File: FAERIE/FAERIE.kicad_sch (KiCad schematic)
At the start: 35 parts, among them J1 UV Sensor, J10 12V IN, J11 Batt IN, J2 UV Bulb, J3 Sparkmax PWM, J4 Sparkmax, J5 Laser1, J7 CAN, J8 CAM1, J9 CAM2, Q1 SSM3K329R_LF, U1 D24V22Fx, U2 TJA1051T-3

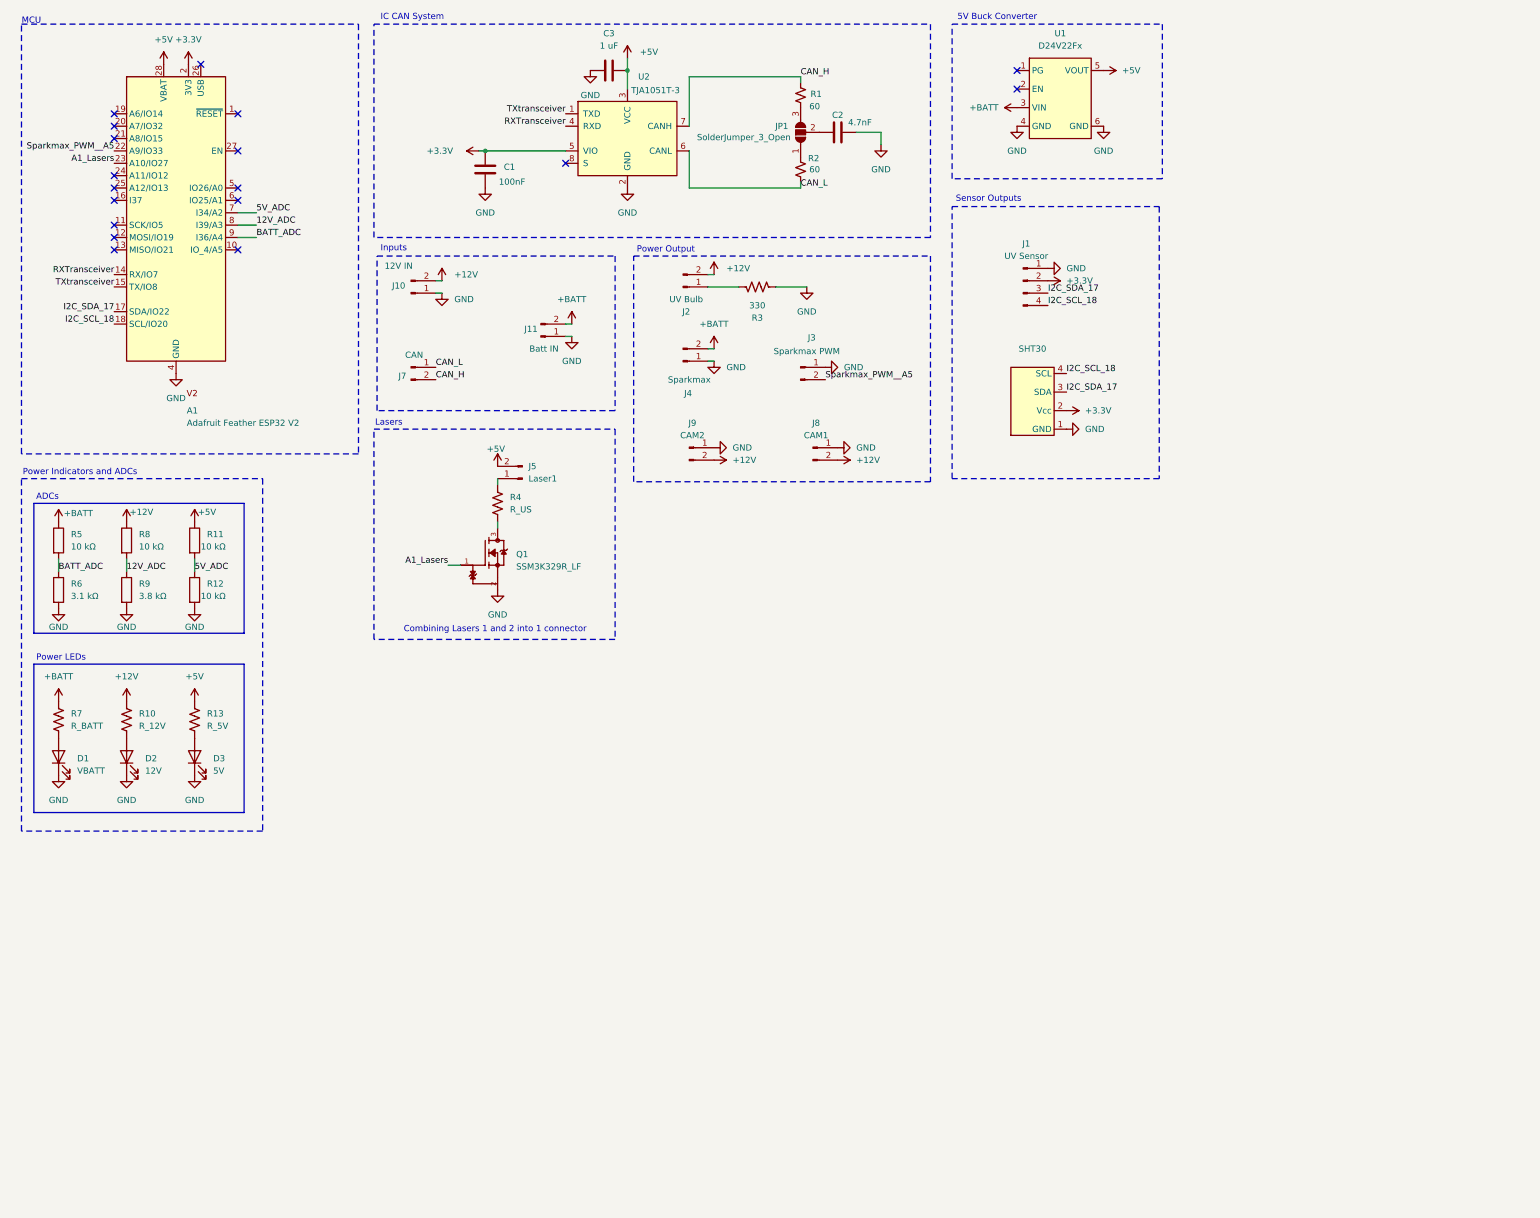
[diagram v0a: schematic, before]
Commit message: FAERIE 2026 V1
FAERIE April 15, 2026
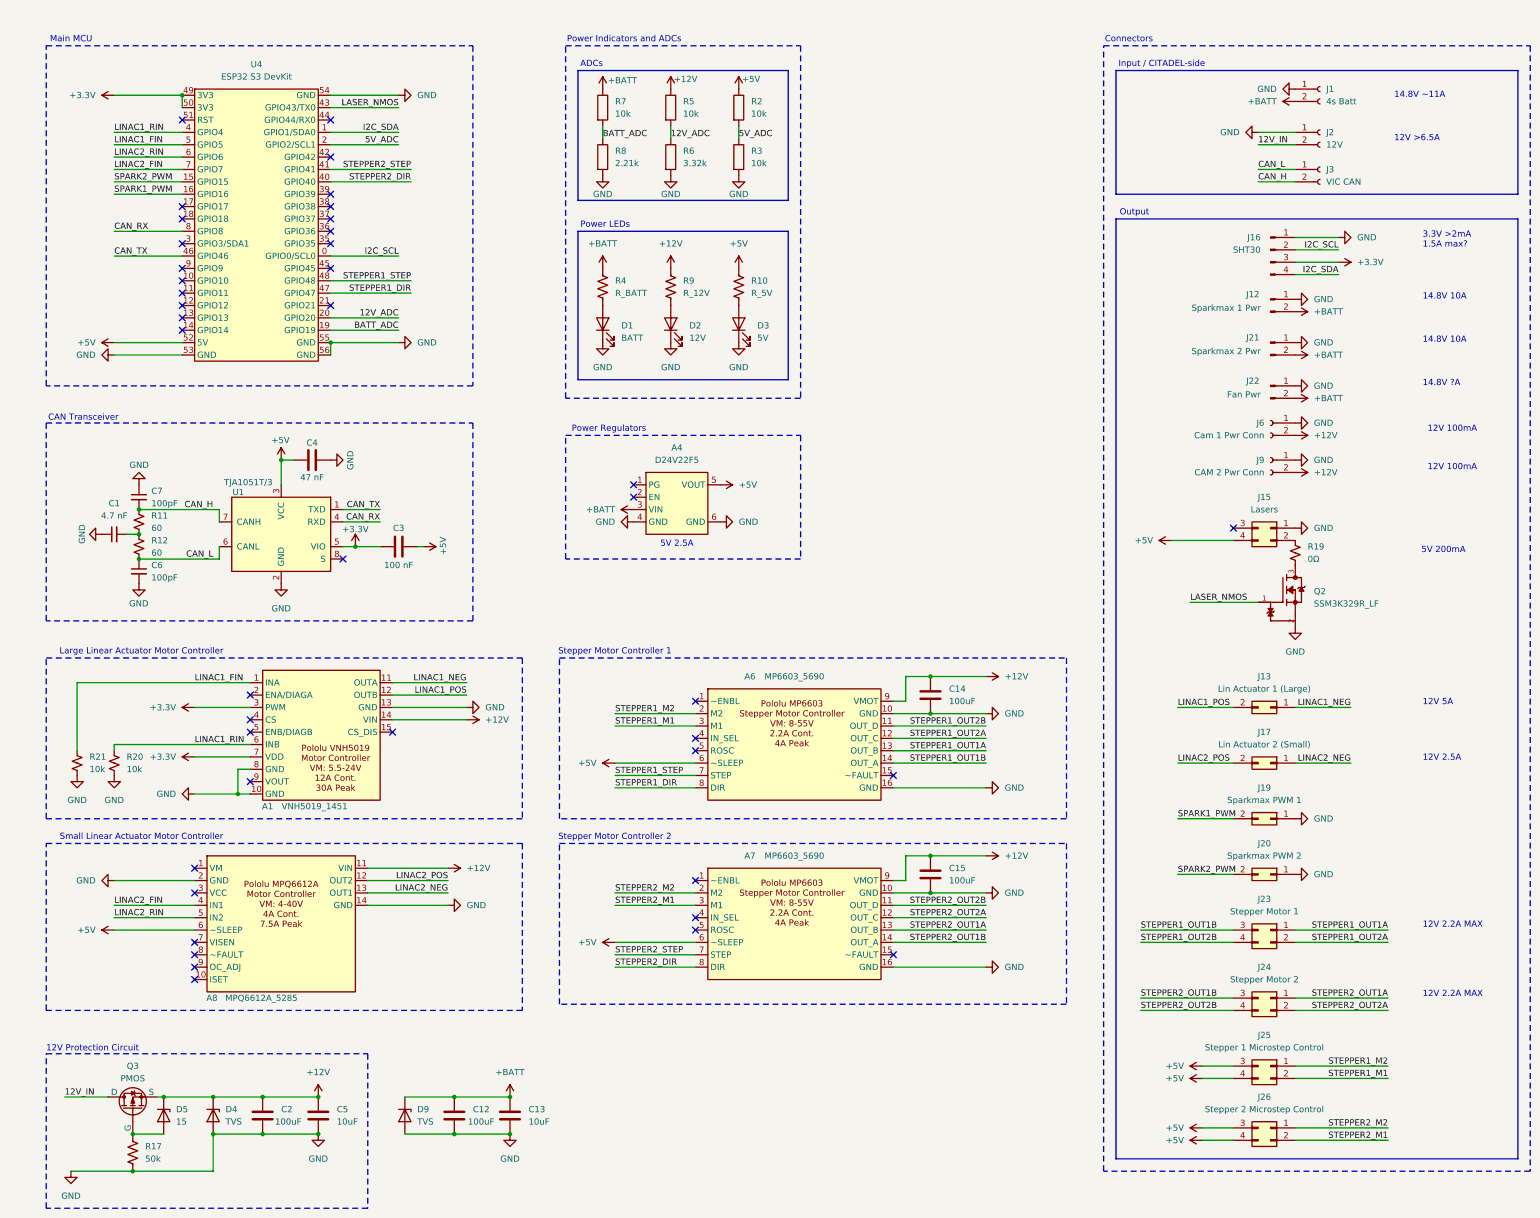
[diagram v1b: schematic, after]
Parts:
- removed A1: Adafruit Feather ESP32 V2, Module:Adafruit_Feather, symbol adafruit_feather_esp32_v2:Adafruit_Feather_ESP32_V2
- removed C1: 100nF, Capacitor_SMD:C_0603_1608Metric_Pad1.08x0.95mm_HandSolder, symbol Device:C
- removed J1: UV Sensor, Connector_Molex:Molex_Mini-Fit_Jr_5566-04A_2x02_P4.20mm_Vertical, symbol Connector:Conn_01x04_Pin
- removed J10: 12V IN, Connector_AMASS:AMASS_XT30PW-M_1x02_P2.50mm_Horizontal, symbol Connector:Conn_01x02_Pin
- removed J11: Batt IN, Connector_AMASS:AMASS_XT60PW-M_1x02_P7.20mm_Horizontal, symbol Connector:Conn_01x02_Pin
- removed J2: UV Bulb, Connector_Molex:Molex_Mini-Fit_Jr_5566-02A_2x01_P4.20mm_Vertical, symbol Connector:Conn_01x02_Pin
- removed J3: Sparkmax PWM, Connector_Molex:Molex_Mini-Fit_Jr_5566-02A_2x01_P4.20mm_Vertical, symbol Connector:Conn_01x02_Pin
- removed J4: Sparkmax, Connector_AMASS:AMASS_XT60PW-F_1x02_P7.20mm_Horizontal, symbol Connector:Conn_01x02_Pin
- removed J5: Laser1, Connector_Molex:Molex_Mini-Fit_Jr_5566-02A_2x01_P4.20mm_Vertical, symbol Connector:Conn_01x02_Pin
- removed J7: CAN, Connector_AMASS:AMASS_XT30PW-F_1x02_P2.50mm_Horizontal, symbol Connector:Conn_01x02_Pin
- removed J8: CAM1, Core_fp:XT30M_MODIFIED, symbol Connector:Conn_01x02_Pin
- removed J9: CAM2, Core_fp:XT30M_MODIFIED, symbol Connector:Conn_01x02_Pin
- removed JP1: SolderJumper_3_Open, Jumper:SolderJumper-3_P1.3mm_Open_Pad1.0x1.5mm_NumberLabels, symbol Jumper:SolderJumper_3_Open
- removed Q1: SSM3K329R_LF, Core_fp:SOTFL95P240X88-3N, symbol SSM3K329R_LF:SSM3K329R_LF
- removed R1, R2: 60, Resistor_SMD:R_0603_1608Metric_Pad0.98x0.95mm_HandSolder, symbol Device:R_Small_US
- removed R11, R12: 10 kΩ, Resistor_SMD:R_0603_1608Metric_Pad0.98x0.95mm_HandSolder, symbol Device:R
- removed R13: R_5V, Resistor_SMD:R_0603_1608Metric_Pad0.98x0.95mm_HandSolder, symbol Device:R_US
- removed R3: 330, Resistor_SMD:R_0603_1608Metric_Pad0.98x0.95mm_HandSolder, symbol Device:R_US
- removed R7: R_BATT, Resistor_SMD:R_0603_1608Metric_Pad0.98x0.95mm_HandSolder, symbol Device:R_US
- removed R9: 3.8 kΩ, Resistor_SMD:R_0603_1608Metric_Pad0.98x0.95mm_HandSolder, symbol Device:R
- removed SHT30: ~, Connector_Molex:Molex_Mini-Fit_Jr_5566-04A_2x02_P4.20mm_Vertical, symbol FAERIESYMBOLS:SHT30
- removed U1: D24V22Fx, Core_fp:D24V22Fx, symbol Core_sym:D24V22Fx
- removed U2: TJA1051T-3, Package_SO:SOIC-8_3.9x4.9mm_P1.27mm, symbol Interface_CAN_LIN:TJA1051T-3
- added A1: VNH5019_1451, FAERIE:VNH5019_1451, symbol Polulu:VNH5019_1451
- added A4: D24V22F5, FAERIE:D24V22Fx, symbol D24V22Fx:D24V22Fx
- added A6, A7: MP6603_5690, FAERIE:MP6603-5690, symbol Polulu:MP6603_5690
- added A8: MPQ6612A_5285, FAERIE:MPQ6612A_5285, symbol Polulu:MPQ6612A_5285
- added C1: 4.7 nF, Capacitor_SMD:C_0603_1608Metric_Pad1.08x0.95mm_HandSolder, symbol Device:C_Small
- added C12, C14, C15: 100uF, Capacitor_SMD:C_1210_3225Metric_Pad1.33x2.70mm_HandSolder, symbol Device:C
- added C13, C5: 10uF, Capacitor_SMD:C_0603_1608Metric_Pad1.08x0.95mm_HandSolder, symbol Device:C
- added C4: 47 nF, Capacitor_SMD:C_0603_1608Metric_Pad1.08x0.95mm_HandSolder, symbol Device:C
- added C6, C7: 100pF, Capacitor_SMD:C_0603_1608Metric_Pad1.08x0.95mm_HandSolder, symbol Device:C_Small
- added D4, D9: TVS, FAERIE:SOD-323HEUS2H_TOS, symbol Device:D_Zener
- added D5: 15, Diode_SMD:D_SOD-123, symbol Device:D_Zener
- added J1: 4s Batt, Connector_AMASS:AMASS_XT60PW-M_1x02_P7.20mm_Horizontal, symbol Connector:Conn_01x02_Socket
- added J12: Sparkmax 1 Pwr, Connector_AMASS:AMASS_XT60PW-F_1x02_P7.20mm_Horizontal, symbol Connector:Conn_01x02_Pin
- added J13: Lin Actuator 1 (Large), Connector_AMASS:AMASS_XT30U-F_1x02_P5.0mm_Vertical, symbol Connector_Generic:Conn_02x01
- added J15: Lasers, Connector_Molex:Molex_Mini-Fit_Jr_5566-04A_2x02_P4.20mm_Vertical, symbol Connector_Generic:Conn_02x02_Top_Bottom
- added J16: SHT30, Connector_Molex:Molex_Mini-Fit_Jr_5566-04A_2x02_P4.20mm_Vertical, symbol Connector:Conn_01x04_Pin
- added J17: Lin Actuator 2 (Small), Connector_AMASS:AMASS_XT30U-F_1x02_P5.0mm_Vertical, symbol Connector_Generic:Conn_02x01
- added J19: Sparkmax PWM 1, Connector_AMASS:AMASS_XT30U-F_1x02_P5.0mm_Vertical, symbol Connector_Generic:Conn_02x01
- added J2: 12V, Connector_AMASS:AMASS_XT30PW-M_1x02_P2.50mm_Horizontal, symbol Connector:Conn_01x02_Socket
- added J20: Sparkmax PWM 2, Connector_AMASS:AMASS_XT30U-F_1x02_P5.0mm_Vertical, symbol Connector_Generic:Conn_02x01
- added J21: Sparkmax 2 Pwr, Connector_AMASS:AMASS_XT60PW-F_1x02_P7.20mm_Horizontal, symbol Connector:Conn_01x02_Pin
- added J22: Fan Pwr, Connector_AMASS:AMASS_XT60PW-F_1x02_P7.20mm_Horizontal, symbol Connector:Conn_01x02_Pin
- added J23: Stepper Motor 1, Connector_Molex:Molex_Mini-Fit_Jr_5566-04A_2x02_P4.20mm_Vertical, symbol Connector_Generic:Conn_02x02_Top_Bottom
- added J24: Stepper Motor 2, Connector_Molex:Molex_Mini-Fit_Jr_5566-04A_2x02_P4.20mm_Vertical, symbol Connector_Generic:Conn_02x02_Top_Bottom
- added J25: Stepper 1 Microstep Control, Connector_PinHeader_2.54mm:PinHeader_2x02_P2.54mm_Vertical, symbol Connector_Generic:Conn_02x02_Top_Bottom
- added J26: Stepper 2 Microstep Control, Connector_PinHeader_2.54mm:PinHeader_2x02_P2.54mm_Vertical, symbol Connector_Generic:Conn_02x02_Top_Bottom
- added J3: VIC CAN, Connector_AMASS:AMASS_XT30PW-F_1x02_P2.50mm_Horizontal, symbol Connector:Conn_01x02_Socket
- added J6: Cam 1 Pwr Conn, Connector_AMASS:AMASS_XT30U-F_1x02_P5.0mm_Vertical, symbol Connector:Conn_01x02_Socket
- added J9: CAM 2 Pwr Conn, Connector_AMASS:AMASS_XT30U-F_1x02_P5.0mm_Vertical, symbol Connector:Conn_01x02_Socket
- added Q2: SSM3K329R_LF, FAERIE:SOT-23F_TOS, symbol SSM3K329R_LF:SSM3K329R_LF
- added Q3: PMOS, Package_TO_SOT_SMD:TO-252-2, symbol Simulation_SPICE:PMOS
- added R11, R12: 60, Resistor_SMD:R_0603_1608Metric_Pad0.98x0.95mm_HandSolder, symbol Device:R_Small_US
- added R17: 50k, Resistor_SMD:R_0603_1608Metric_Pad0.98x0.95mm_HandSolder, symbol Device:R_US
- added R19: 0Ω, Resistor_SMD:R_0603_1608Metric_Pad0.98x0.95mm_HandSolder, symbol Device:R_Small_US
- added R2, R3, R7: 10k, Resistor_SMD:R_0603_1608Metric_Pad0.98x0.95mm_HandSolder, symbol Device:R
- added R20, R21: 10k, Resistor_SMD:R_0603_1608Metric_Pad0.98x0.95mm_HandSolder, symbol Device:R_Small_US
- added R9: R_12V, Resistor_SMD:R_0603_1608Metric_Pad0.98x0.95mm_HandSolder, symbol Device:R_US
- added U1: TJA1051T/3, Package_SO:SOIC-8_3.9x4.9mm_P1.27mm, symbol Interface_CAN_LIN:TJA1051T-3
- added U4: ESP32 S3 DevKit, FAERIE:ESP32-S3-DevKit_No_Keep-Out_Zone, symbol SANXIXING:ESP32_S3_Dev_Board
- C2: value 4.7nF -> 100uF; footprint Capacitor_SMD:C_0603_1608Metric_Pad1.08x0.95mm_HandSolder -> Capacitor_SMD:C_1210_3225Metric_Pad1.33x2.70mm_HandSolder
- C3: value 1 uF -> 100 nF
- D1: value VBATT -> BATT
- R10: value R_12V -> R_5V
- R4: value R_US -> R_BATT
- R5: value 10 kΩ -> 10k
- R6: value 3.1 kΩ -> 3.32k
- R8: value 10 kΩ -> 2.21k
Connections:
- net +12V: now also C2.1, R5.1, A1.14 (VIN), A6.9 (VMOT), A7.9 (VMOT), A8.11 (VIN), C14.1, C15.1, C5.1, D4.1 (K), D5.1 (K), J6.2 (Pin_2), J9.2 (Pin_2), Q3.3 (S), R9.1; no longer R10.1, R8.1
- net +3.3V: now also C3.2, A1.3 (PWM), A1.7 (VDD), J16.3 (Pin_3), U1.5 (VIO), U4.49 (3V3), U4.50 (3V3)
- net +5V: now also R10.1, A4.5 (VOUT), A6.6 (~SLEEP), A7.6 (~SLEEP), A8.6 (~SLEEP), C4.1, J15.4 (Pin_4), J25.3 (Pin_3), J25.4 (Pin_4), J26.3 (Pin_3), J26.4 (Pin_4), R2.1, U1.3 (VCC), U4.52 (5V)
- net +BATT: now also R4.1, A4.3 (VIN), C12.1, C13.1, D9.1 (K), J1.2 (Pin_2), J12.2 (Pin_2), J21.2 (Pin_2), J22.2 (Pin_2), R7.1; no longer R5.1
- net 12V_ADC: now also R5.2, R6.1, U4.20 (GPIO20); no longer R8.2
- net 5V_ADC: now also R2.2, R3.1, U4.2 (GPIO2/SCL1)
- net BATT_ADC: now also R8.1, R7.2, U4.19 (GPIO19); no longer R5.2, R6.1
- net CAN_H: now also C7.2, J3.2 (Pin_2), R11.1, U1.7 (CANH)
- net CAN_L: now also C6.1, J3.1 (Pin_1), R12.2, U1.6 (CANL)
- net GND: now also R8.2, A1.10 (GND), A1.13 (GND), A1.8 (GND), A4.4 (GND), A4.6 (GND), A6.10 (GND), A6.16 (GND), A7.10 (GND), A7.16 (GND), A8.14 (GND), A8.2 (GND), C1.1, C12.2, C13.2, C14.2, C15.2, C4.2, C5.2, C6.2, C7.1, D4.2 (A), D9.2 (A), J1.1 (Pin_1), J12.1 (Pin_1), J15.1 (Pin_1), J16.1 (Pin_1), J19.1 (Pin_1), J2.1 (Pin_1), J20.1 (Pin_1), J21.1 (Pin_1), J22.1 (Pin_1), J6.1 (Pin_1), J9.1 (Pin_1), Q2.2, R17.2, R20.1, R21.1, R3.2, U1.2 (GND), U4.53 (GND), U4.54 (GND), U4.55 (GND), U4.56 (GND); no longer C3.2
- net at D1.2 (A): now also R4.2
- net at D2.2 (A): now also R9.2; no longer R10.2
- net at D3.2 (A): now also R10.2
- new net: Q2.3, R19.2
- new net: J15.2 (Pin_2), R19.1
- new net: D5.2 (A), Q3.2 (G), R17.1
- new net: C1.2, R11.2, R12.1
- new net 12V_IN: J2.2 (Pin_2), Q3.1 (D)
- new net CAN_RX: U1.4 (RXD), U4.8 (GPIO8)
- new net CAN_TX: U1.1 (TXD), U4.46 (GPIO46)
- new net I2C_SCL: J16.2 (Pin_2), U4.0 (GPIO0/SCL0)
- new net I2C_SDA: J16.4 (Pin_4), U4.1 (GPIO1/SDA0)
- new net LASER_NMOS: Q2.1, U4.43 (GPIO43/TX0)
- new net LINAC1_FIN: A1.1 (INA), R21.2, U4.5 (GPIO5)
- new net LINAC1_NEG: A1.11 (OUTA), J13.1 (Pin_1)
- new net LINAC1_POS: A1.12 (OUTB), J13.2 (Pin_2)
- new net LINAC1_RIN: A1.6 (INB), R20.2, U4.4 (GPIO4)
- new net LINAC2_FIN: A8.4 (IN1), U4.7 (GPIO7)
- new net LINAC2_NEG: A8.13 (OUT1), J17.1 (Pin_1)
- new net LINAC2_POS: A8.12 (OUT2), J17.2 (Pin_2)
- new net LINAC2_RIN: A8.5 (IN2), U4.6 (GPIO6)
- new net SPARK1_PWM: J19.2 (Pin_2), U4.16 (GPIO16)
- new net SPARK2_PWM: J20.2 (Pin_2), U4.15 (GPIO15)
- new net STEPPER1_DIR: A6.8 (DIR), U4.47 (GPIO47)
- new net STEPPER1_M1: A6.3 (M1), J25.2 (Pin_2)
- new net STEPPER1_M2: A6.2 (M2), J25.1 (Pin_1)
- new net STEPPER1_OUT1A: A6.13 (OUT_B), J23.1 (Pin_1)
- new net STEPPER1_OUT1B: A6.14 (OUT_A), J23.3 (Pin_3)
- new net STEPPER1_OUT2A: A6.12 (OUT_C), J23.2 (Pin_2)
- new net STEPPER1_OUT2B: A6.11 (OUT_D), J23.4 (Pin_4)
- new net STEPPER1_STEP: A6.7 (STEP), U4.48 (GPIO48)
- new net STEPPER2_DIR: A7.8 (DIR), U4.40 (GPIO40)
- new net STEPPER2_M1: A7.3 (M1), J26.2 (Pin_2)
- new net STEPPER2_M2: A7.2 (M2), J26.1 (Pin_1)
- new net STEPPER2_OUT1A: A7.13 (OUT_B), J24.1 (Pin_1)
- new net STEPPER2_OUT1B: A7.14 (OUT_A), J24.3 (Pin_3)
- new net STEPPER2_OUT2A: A7.12 (OUT_C), J24.2 (Pin_2)
- new net STEPPER2_OUT2B: A7.11 (OUT_D), J24.4 (Pin_4)
- new net STEPPER2_STEP: A7.7 (STEP), U4.41 (GPIO41)
- no-connect marks 18 -> 42
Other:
- note added: "12V 100mA"
- note added: "12V 2.2A MAX"
- note added: "12V 2.5A"
- note added: "12V 5A"
- note added: "12V >6.5A"
- note added: "12V Protection Circuit"
- note added: "14.8V 10A"
- note added: "14.8V ?A"
- note added: "14.8V ~11A"
- note added: "3.3V >2mA 1.5A max?"
- note added: "5V 2.5A"
- note added: "5V 200mA"
- note added: "CAN Transceiver"
- note added: "Connectors"
- note added: "Input / CITADEL-side"
- note added: "Large Linear Actuator Motor Controller"
- note added: "Main MCU"
- note added: "Output"
- note added: "Power Regulators"
- note added: "Small Linear Actuator Motor Controller"
- note added: "Stepper Motor Controller 1"
- note added: "Stepper Motor Controller 2"
- note removed: "5V Buck Converter"
- note removed: "Combining Lasers 1 and 2 into 1 connector"
- note removed: "IC CAN System"
- note removed: "Inputs"
- note removed: "Lasers"
- note removed: "MCU"
- note removed: "Power Output"
- note removed: "Sensor Outputs"
- company: (none) -> UAH SHC ASTRA
- title: (none) -> FAERIE ESP32 2026

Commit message: FAERIE 2026 r1.01
Changed Sparkmax PWM 1 and 2 from XT-30 connectors to Molex
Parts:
- J19, J20: footprint Connector_AMASS:AMASS_XT30U-F_1x02_P5.0mm_Vertical -> Connector_Molex:Molex_Mini-Fit_Jr_5566-02A_2x01_P4.20mm_Vertical
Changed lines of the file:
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@@
 	(title_block
 		(title "FAERIE ESP32 2026")
-		(date "2026-04-15")
-		(rev "1.0")
+		(date "2026-04-21")
+		(rev "1.01")
 		(company "UAH SHC ASTRA")
 		(comment 1 "Created by Robert Geren")
@@
 			)
 		)
-		(property "Footprint" "Connector_AMASS:AMASS_XT30U-F_1x02_P5.0mm_Vertical"
+		(property "Footprint" "Connector_Molex:Molex_Mini-Fit_Jr_5566-02A_2x01_P4.20mm_Vertical"
 			(at 271.78 190.5 0)
 			(effects
@@
 			)
 		)
-		(property "Footprint" "Connector_AMASS:AMASS_XT30U-F_1x02_P5.0mm_Vertical"
+		(property "Footprint" "Connector_Molex:Molex_Mini-Fit_Jr_5566-02A_2x01_P4.20mm_Vertical"
 			(at 271.78 179.07 0)
 			(effects
